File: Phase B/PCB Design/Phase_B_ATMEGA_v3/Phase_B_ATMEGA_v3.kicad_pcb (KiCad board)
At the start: 2 copper layers, 82.5 x 76.2 mm, 49 parts, among them J1 AVR-ISP-6, J2 USB_B_Mini, J3 ESP_Conn, U1 CA56-12EWA, U2 74HC595, U3 ATmega32U4-A, U4 USBLC6-2SC6, U5 LP2985-3.3, Y1 16MHz

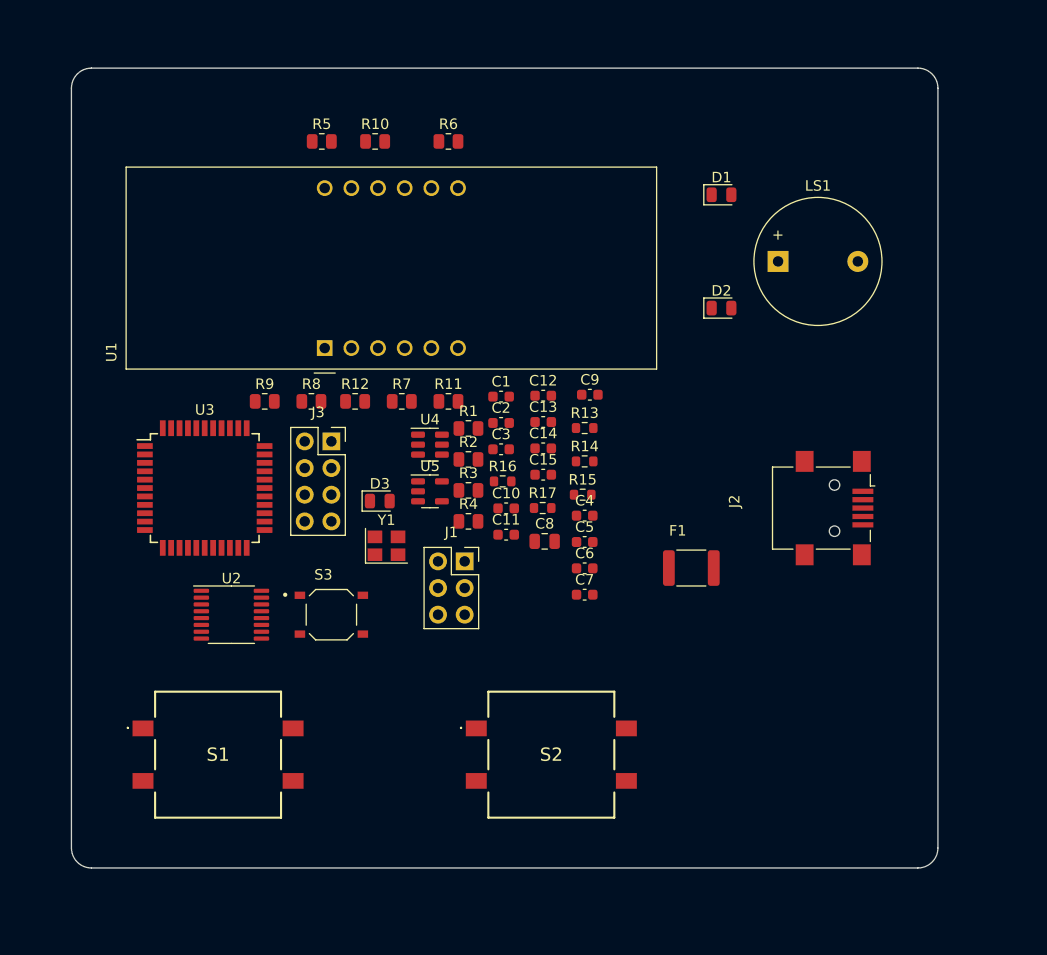
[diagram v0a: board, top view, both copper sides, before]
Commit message: PCB Final Design as well as plot, gerber, and BOM updates
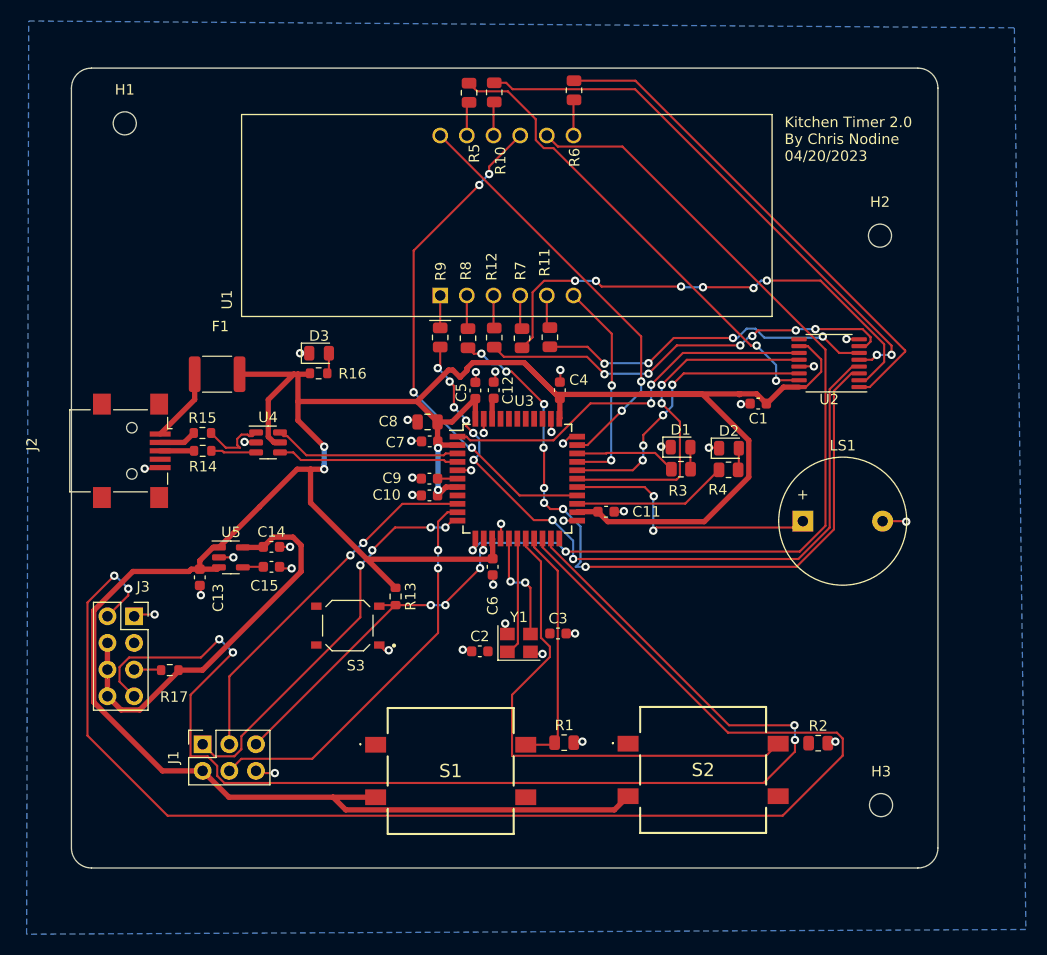
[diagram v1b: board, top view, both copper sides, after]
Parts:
- added H1: MountingHole, MountingHole:MountingHole_2.2mm_M2, F.Cu at (133.3, 33.2)
- added H2: MountingHole, MountingHole:MountingHole_2.2mm_M2, F.Cu at (205.3, 43.9)
- added H3: MountingHole, MountingHole:MountingHole_2.2mm_M2, F.Cu at (205.4, 98.2)
- moved J2 67.2 mm to (134.0, 64.4)
- moved U2 61.8 mm to (200.4, 56.0), turned to 180 degrees
- moved F1 48.8 mm to (142.2, 57.1)
- moved R2 42.9 mm to (199.4, 92.2)
- moved R17 38.7 mm to (137.6, 85.3), turned to 180 degrees
- moved R15 36.7 mm to (140.8, 62.7)
- moved R14 36.4 mm to (140.8, 64.4)
- moved C13 35.9 mm to (140.5, 76.5), turned to -90 degrees
- moved R1 31.3 mm to (175.2, 92.2)
- moved J1 30.4 mm to (140.8, 92.3), turned to 90 degrees
- moved U3 29.8 mm to (170.8, 67.0)
- moved C14 27.5 mm to (147.3, 73.5)
- moved C15 27.3 mm to (147.3, 75.5)
- moved R4 25.3 mm to (190.9, 66.2)
- moved J3 25.1 mm to (134.2, 80.2)
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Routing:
- net +5V: track 0.00 -> 272.3 mm, vias 0 -> 4
- net TX: track 0.00 -> 137.7 mm, vias 0 -> 2
- net RX: track 0.00 -> 121.4 mm, vias 0 -> 4
- net Dig3: track 0.00 -> 88.3 mm, vias 0 -> 2
- net d: track 0.00 -> 69.7 mm, vias 0 -> 8
- net e: track 0.00 -> 69.7 mm, vias 0 -> 8
- net f: track 0.00 -> 52.4 mm, vias 0 -> 2
- net Button_2: track 0.00 -> 49.0 mm
- net Dig2: track 0.00 -> 48.3 mm, vias 0 -> 4
- net b: track 0.00 -> 48.1 mm
- net c: track 0.00 -> 47.6 mm, vias 0 -> 6
- net a: track 0.00 -> 45.2 mm, vias 0 -> 2
- net GND: track 0.00 -> 43.7 mm, vias 0 -> 37
- net dp: track 0.00 -> 40.7 mm, vias 0 -> 6
- net Dig1: track 0.00 -> 40.5 mm, vias 0 -> 2
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- added copper zone on B.Cu, net GND
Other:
- board text added: "Kitchen Timer 2.0 By Chris Nodine 04/20/2023"
